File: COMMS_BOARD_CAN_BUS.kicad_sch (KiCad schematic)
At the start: 8 parts, among them IC1 TCAN1044VDDFR, J5 Conn_01x02

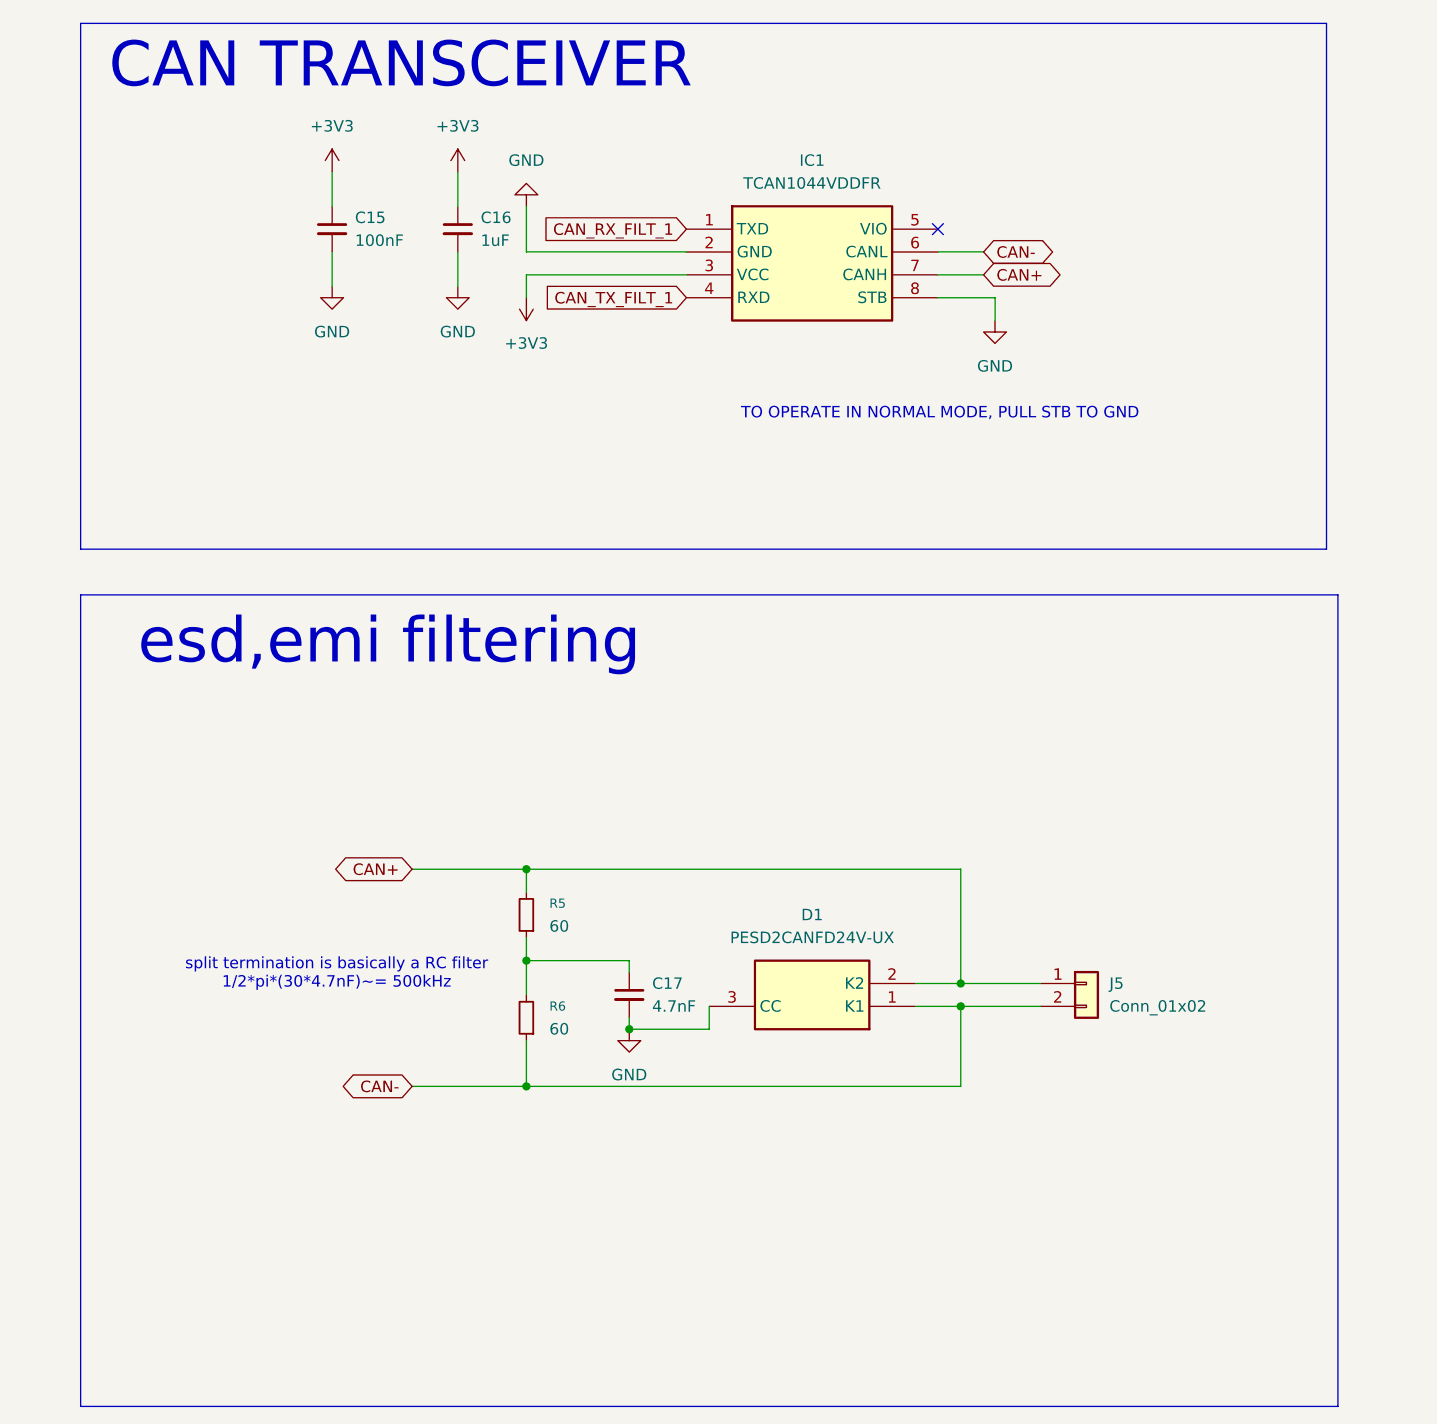
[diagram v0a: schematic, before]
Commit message: ADDE IMU
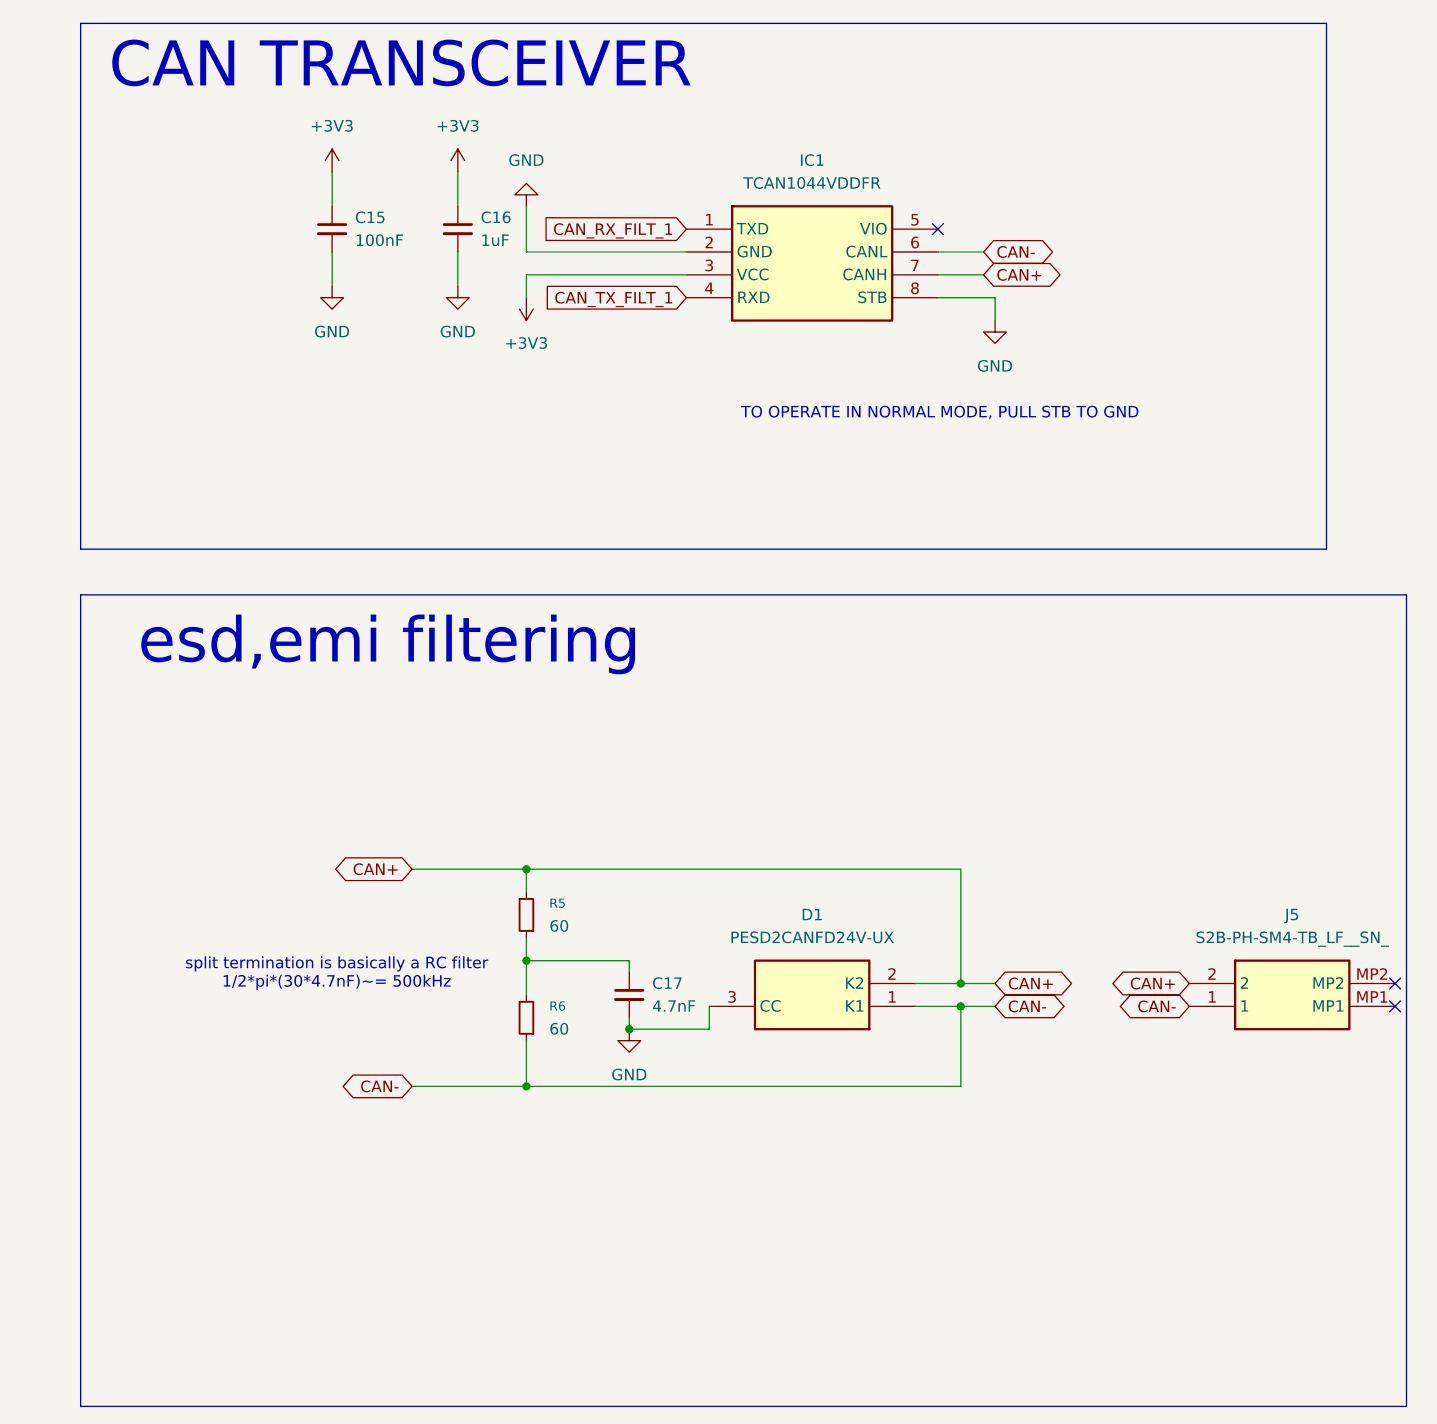
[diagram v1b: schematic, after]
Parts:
- removed J5: Conn_01x02, Connector_JST:JST_XH_B2B-XH-A_1x02_P2.50mm_Vertical, symbol Connector_Generic:Conn_01x02
- added J5: S2B-PH-SM4-TB_LF__SN_, SamacSys_Parts:S2BPHSM4TBLFSN, symbol Samac_sys:S2B-PH-SM4-TB_LF__SN_
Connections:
- net CAN+: now also J5.2
- net CAN-: now also J5.1
- no-connect marks 1 -> 3
